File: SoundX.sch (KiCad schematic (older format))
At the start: 51 parts, among them CN1 EDGE_CONN, CN2 RAW_AUDIO_OUT, CN3 CONN_MIDI_IN, CN4 CONN_MIDI_OUT, U1 GAL20V8, U2 MOS_6551_ACIA, U3 YM3526, U4 6N138, U6 YM3014, U7 LM324, Y1 3.579545 MHz, Y2 3M

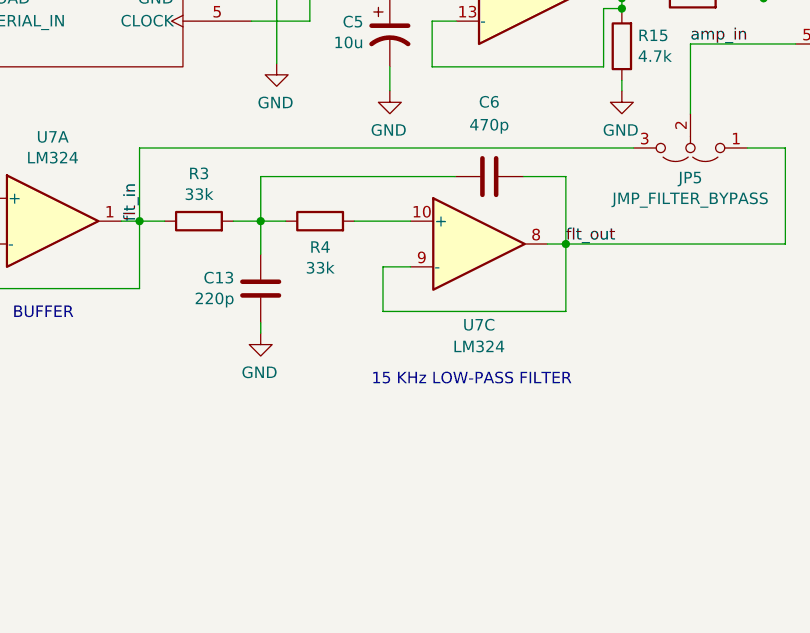
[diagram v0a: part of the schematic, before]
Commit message: Fix C13 - Thanks TLC!
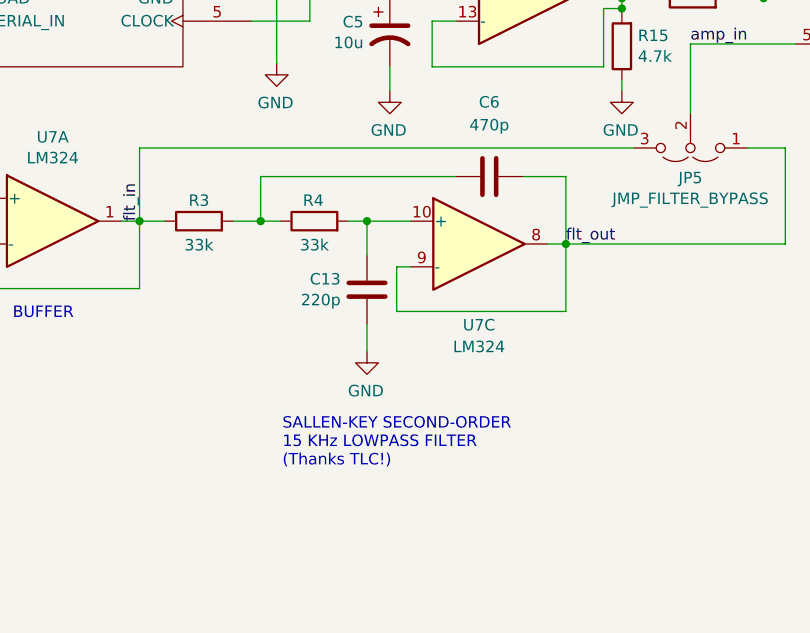
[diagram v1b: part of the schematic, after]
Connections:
- net at C6.1, R3.2, R4.1: no longer C13.1
- net at R4.2, U7.10 (+): now also C13.1
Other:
- note added: "SALLEN-KEY SECOND-ORDER\n15 KHz LOWPASS FILTER\n(Thanks TLC!)"
- note removed: "15 KHz LOW-PASS FILTER"
- moved on the sheet: C13, R4
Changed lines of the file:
@@
 Sheet 1 1
 Title "SoundX"
-Date "2023-08-19"
+Date "2026-07-11"
 Rev "1git"
 Comp "SukkoPera"
 Comment1 "Inspired by the C64 Sound Expander"
-Comment2 ""
+Comment2 "https://github.com/SukkoPera/SoundX"
 Comment3 "Licensed under CC BY-NC-SA 4.0"
 Comment4 ""
@@
 AR Path="/6579482E/693006B1" Ref="R?"  Part="1"
 AR Path="/693006B1" Ref="R3"  Part="1"
-F 0 "R3" V 9882 6270 50  0000 C CNN
-F 1 "33k" V 9791 6270 50  0000 C CNN
+F 0 "R3" V 9765 6270 50  0000 C CNN
+F 1 "33k" V 9570 6270 50  0000 C CNN
 F 2 "Resistor_THT:R_Axial_DIN0207_L6.3mm_D2.5mm_P2.54mm_Vertical" V 9605 6270 50  0001 C CNN
 F 3 "~" H 9675 6270 50  0001 C CNN
@@
 L Device:R R?
 U 1 1 69316664
-P 10205 6270
+P 10180 6270
 AR Path="/6579482E/69316664" Ref="R?"  Part="1"
 AR Path="/69316664" Ref="R4"  Part="1"
-F 0 "R4" V 10090 6270 50  0000 C CNN
-F 1 "33k" V 9999 6270 50  0000 C CNN
-F 2 "Resistor_THT:R_Axial_DIN0207_L6.3mm_D2.5mm_P2.54mm_Vertical" V 10135 6270 50  0001 C CNN
-F 3 "~" H 10205 6270 50  0001 C CNN
-F 4 "OPL" H 10205 6270 50  0001 C CNN "Notes"
-	1    10205 6270
+F 0 "R4" V 10270 6275 50  0000 C CNN
+F 1 "33k" V 10075 6270 50  0000 C CNN
+F 2 "Resistor_THT:R_Axial_DIN0207_L6.3mm_D2.5mm_P2.54mm_Vertical" V 10110 6270 50  0001 C CNN
+F 3 "~" H 10180 6270 50  0001 C CNN
+F 4 "OPL" H 10180 6270 50  0001 C CNN "Notes"
+	1    10180 6270
 	0    -1   -1   0
 $EndComp
@@
 	9825 6270 9945 6270
 Wire Wire Line
-	10355 6270 10600 6270
-Wire Wire Line
-	11280 6665 10480 6665
-Wire Wire Line
-	10480 6665 10480 6470
-Wire Wire Line
-	10480 6470 10600 6470
+	10330 6270 10410 6270
+Wire Wire Line
+	11280 6665 10540 6665
+Wire Wire Line
+	10540 6665 10540 6470
+Wire Wire Line
+	10540 6470 10600 6470
 Wire Wire Line
 	11280 6665 11280 6370
@@
 Connection ~ 9945 6270
 Wire Wire Line
-	9945 6270 10055 6270
+	9945 6270 10030 6270
 $Comp
 L Device:C C?
@@
 Wire Wire Line
 	10795 6075 9945 6075
-Text Notes 10430 6995 0    50   ~ 0
-15 KHz LOW-PASS FILTER
+Text Notes 10040 7350 0    50   ~ 0
+SALLEN-KEY SECOND-ORDER\n15 KHz LOWPASS FILTER\n(Thanks TLC!)
 Text Notes 12390 6035 0    50   ~ 0
 AMPLIFIER
@@
 L Device:C C?
 U 1 1 65814F5E
-P 9945 6565
+P 10410 6570
 AR Path="/6579482E/65814F5E" Ref="C?"  Part="1"
 AR Path="/65814F5E" Ref="C13"  Part="1"
-F 0 "C13" H 9830 6611 50  0000 R CNN
-F 1 "220p" H 9830 6520 50  0000 R CNN
-F 2 "Capacitor_THT:C_Disc_D7.0mm_W2.5mm_P5.00mm" H 9983 6415 50  0001 C CNN
-F 3 "~" H 9945 6565 50  0001 C CNN
-F 4 "" H 9945 6565 50  0001 C CNN "MouserPN"
-F 5 "OPL" H 9945 6565 50  0001 C CNN "Notes"
-	1    9945 6565
-	1    0    0    -1
-$EndComp
-Wire Wire Line
-	9945 6270 9945 6415
+F 0 "C13" H 10295 6616 50  0000 R CNN
+F 1 "220p" H 10295 6525 50  0000 R CNN
+F 2 "Capacitor_THT:C_Disc_D7.0mm_W2.5mm_P5.00mm" H 10448 6420 50  0001 C CNN
+F 3 "~" H 10410 6570 50  0001 C CNN
+F 4 "" H 10410 6570 50  0001 C CNN "MouserPN"
+F 5 "OPL" H 10410 6570 50  0001 C CNN "Notes"
+	1    10410 6570
+	1    0    0    -1
+$EndComp
+Wire Wire Line
+	10410 6270 10410 6420
 $Comp
 L power:GND #PWR010
 U 1 1 65841B0E
-P 9945 6760
-F 0 "#PWR010" H 9945 6510 50  0001 C CNN
-F 1 "GND" H 9950 6587 50  0000 C CNN
-F 2 "" H 9945 6760 50  0001 C CNN
-F 3 "" H 9945 6760 50  0001 C CNN
-	1    9945 6760
+P 10410 6840
+F 0 "#PWR010" H 10410 6590 50  0001 C CNN
+F 1 "GND" H 10415 6667 50  0000 C CNN
+F 2 "" H 10410 6840 50  0001 C CNN
+F 3 "" H 10410 6840 50  0001 C CNN
+	1    10410 6840
 	-1   0    0    -1
 $EndComp
 Wire Wire Line
-	9945 6760 9945 6715
+	10410 6840 10410 6720
 $Comp
 L Device:C C?
@@
 Text Notes 12620 4825 0    50   ~ 0
 VARIABLE GAIN FOR\nTHE LAST AMP STAGE
+Connection ~ 10410 6270
+Wire Wire Line
+	10410 6270 10600 6270
 Wire Bus Line
 	5505 5895 5505 6595
